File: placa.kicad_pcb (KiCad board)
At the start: 2 copper layers, 40 x 40 mm, 74 parts, among them J1 SW, J10 CONN_01X04_Straight, J11 CONN_01X04_Straight, J12 CONN_01X04_Straight, J13 CONN_01X04_Straight, J2 μUSB, J3 BATT, J6 CONN_01X12_Straight, J7 CONN_02X12_Straight, J8 CONN_01X04_Straight, J9 CONN_01X04_Straight, Q1 BSS84, Q2 BSS138P, Q3 BSS138P, U1 AP2112K-3.3TRG1, U2 MCP73831, U3 MIC2253-06YML-TR, U4 ADS1000, U5 LMC7101AIM5, U6 DRV8837, U7 DRV8837, U8 PCA9670

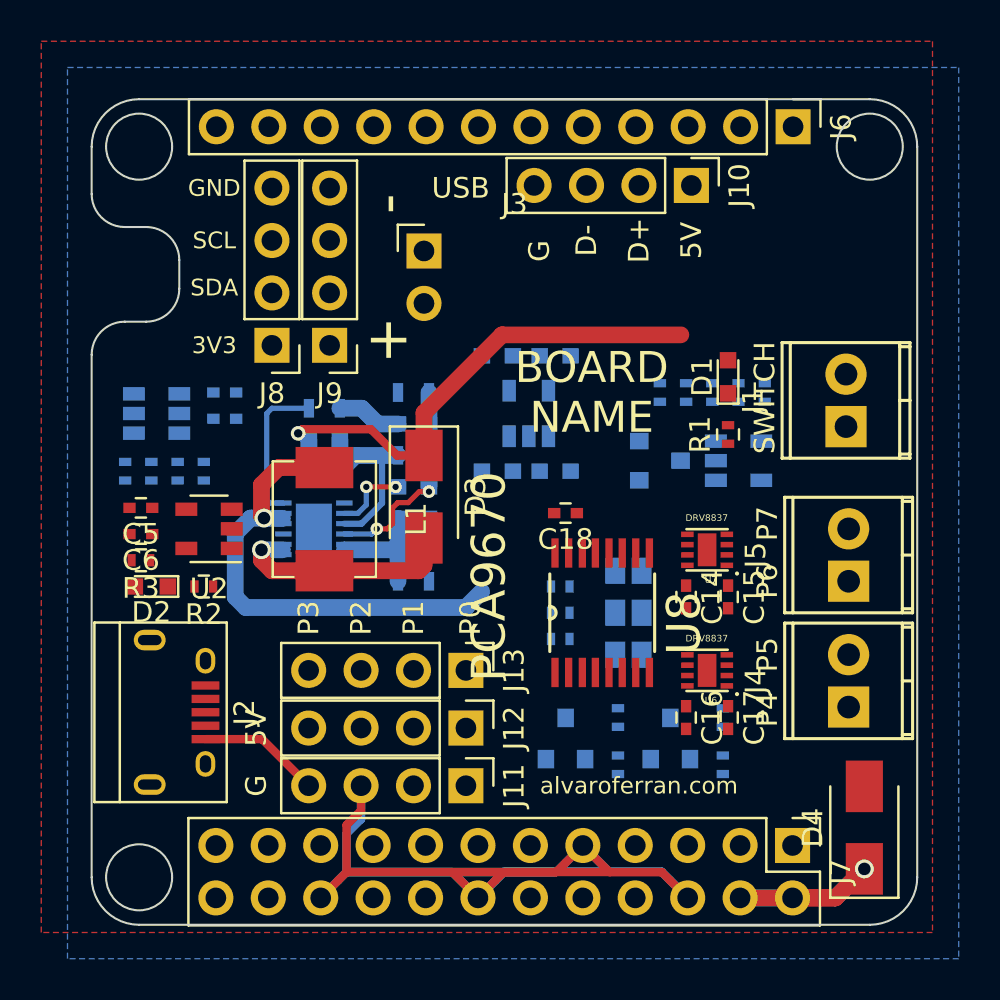
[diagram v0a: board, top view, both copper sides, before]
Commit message: Board
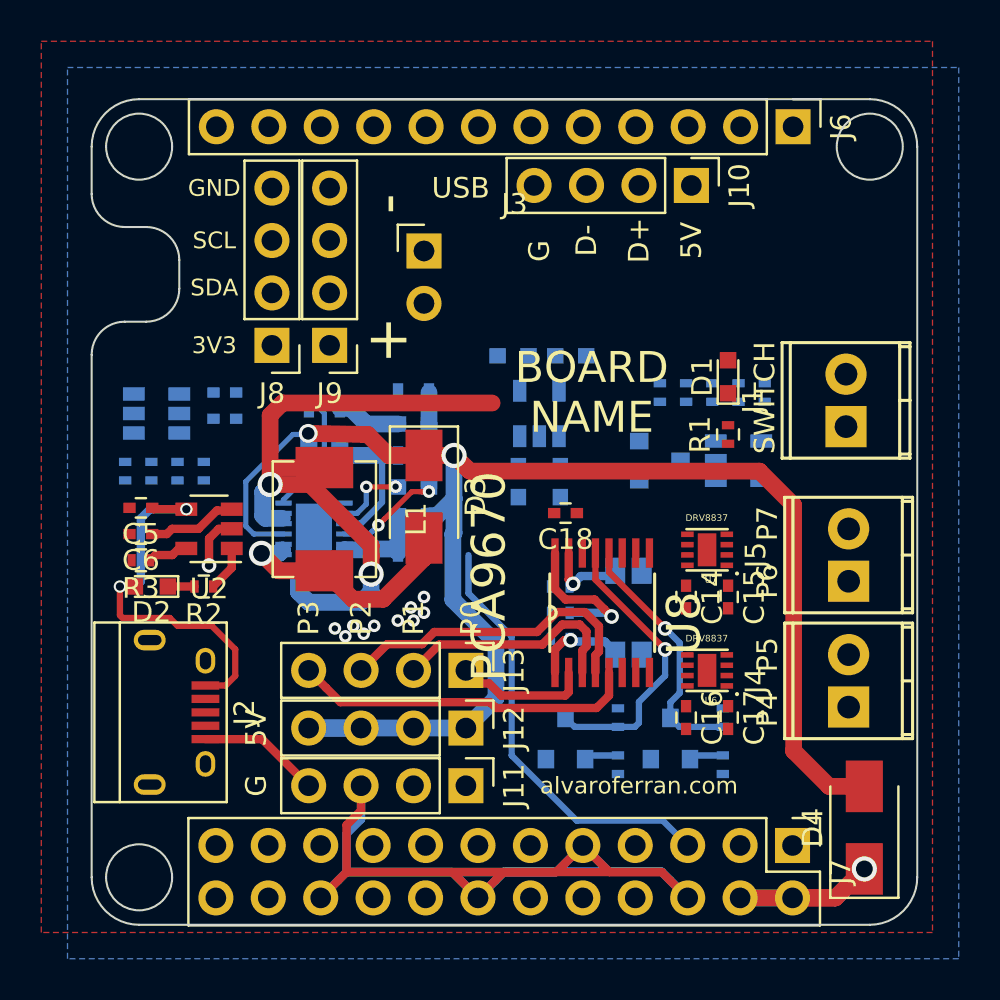
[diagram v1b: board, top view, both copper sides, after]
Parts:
- removed JP2: Jumper_NO, Connectors:GS2
- moved C8 5.71 mm to (159.3, 88.4), turned to 0 degrees
- moved C9 1.65 mm to (164.1, 85.2)
- moved R16 1.40 mm to (164.1, 87.0)
- moved C1 1.14 mm to (169.2, 83.6), turned to 270 degrees
- moved C2 0.76 mm to (168.9, 77.5)
- moved C4 0.76 mm to (171.7, 77.5)
- moved C3 0.57 mm to (171.2, 83.6), turned to 270 degrees
- moved U1 0.51 mm to (170.2, 80.3)
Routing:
- net 5V: track 25.0 -> 77.2 mm, vias 1 -> 2
- net /SCL: track 0.00 -> 20.9 mm
- net Net-(C5-Pad1): track 0.00 -> 19.7 mm, vias 0 -> 2
- net /GPIO3: track 0.00 -> 16.7 mm
- net /GPIO2: track 0.00 -> 15.3 mm
- net /SDAH: track 0.00 -> 14.0 mm, vias 0 -> 1
- net /SCLH: track 0.00 -> 12.3 mm, vias 0 -> 1
- net /GPIO1: track 0.00 -> 11.5 mm
- net VBAT: track 23.7 -> 33.6 mm, vias 1 -> 2
- net Net-(JP2-Pad1): track 0.00 -> 7.15 mm, vias 0 -> 1
- net /GPIO0: track 0.00 -> 6.65 mm
- net Net-(JP3-Pad1): track 0.00 -> 4.58 mm, vias 0 -> 1
- net Net-(C6-Pad1): track 0.00 -> 4.35 mm
- net Net-(JP1-Pad1): track 0.00 -> 3.89 mm, vias 0 -> 1
- net 3.3V: track 0.00 -> 3.33 mm
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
